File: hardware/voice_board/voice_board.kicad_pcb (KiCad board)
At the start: 2 copper layers, 131 parts, among them J1 Conn_02x06_Odd_Even, J10 Conn_01x02_Male, J2 Conn_02x02_Odd_Even, J3 Conn_02x02_Odd_Even, J4 Conn_01x02_Male, J5 Conn_02x03_Odd_Even, J6 Conn_02x02_Odd_Even, J7 Conn_02x02_Odd_Even, J8 Conn_02x02_Odd_Even, J9 Conn_02x02_Odd_Even, Q1 BC327, Q10 BC557, Q11 BC557, Q12 BC557, Q13 BC557, Q14 BC557, Q15 BC557, Q16 BC557, Q17 BC547, Q18 BC547, Q19 2N7000, Q2 BC557, Q20 2N7000, Q21 BC547, Q22 BC547, Q3 BC327, Q4 BC557, Q5 BC557, Q6 BC557, Q7 BC557, Q8 BC557, Q9 BC557, U1 TL074, U2 MCP4822, U3 LM324

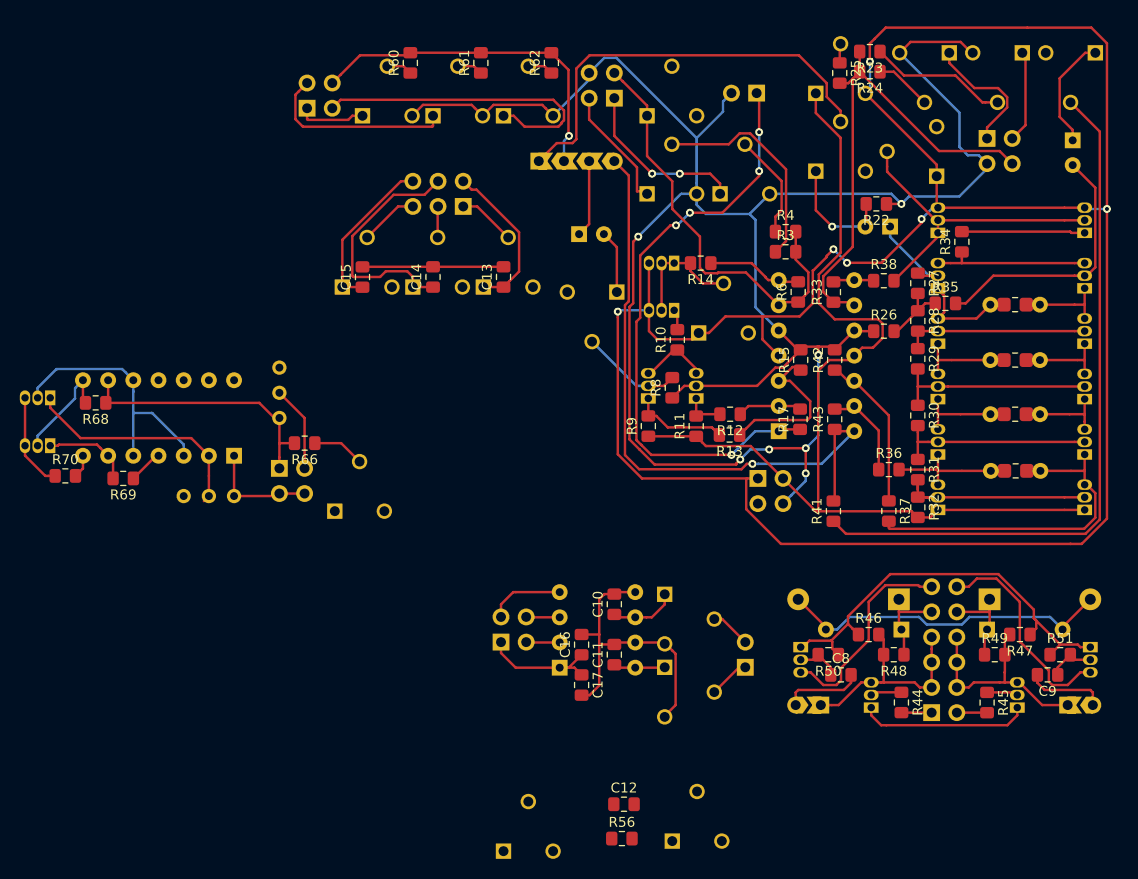
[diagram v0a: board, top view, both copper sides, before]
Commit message: silk screen final?
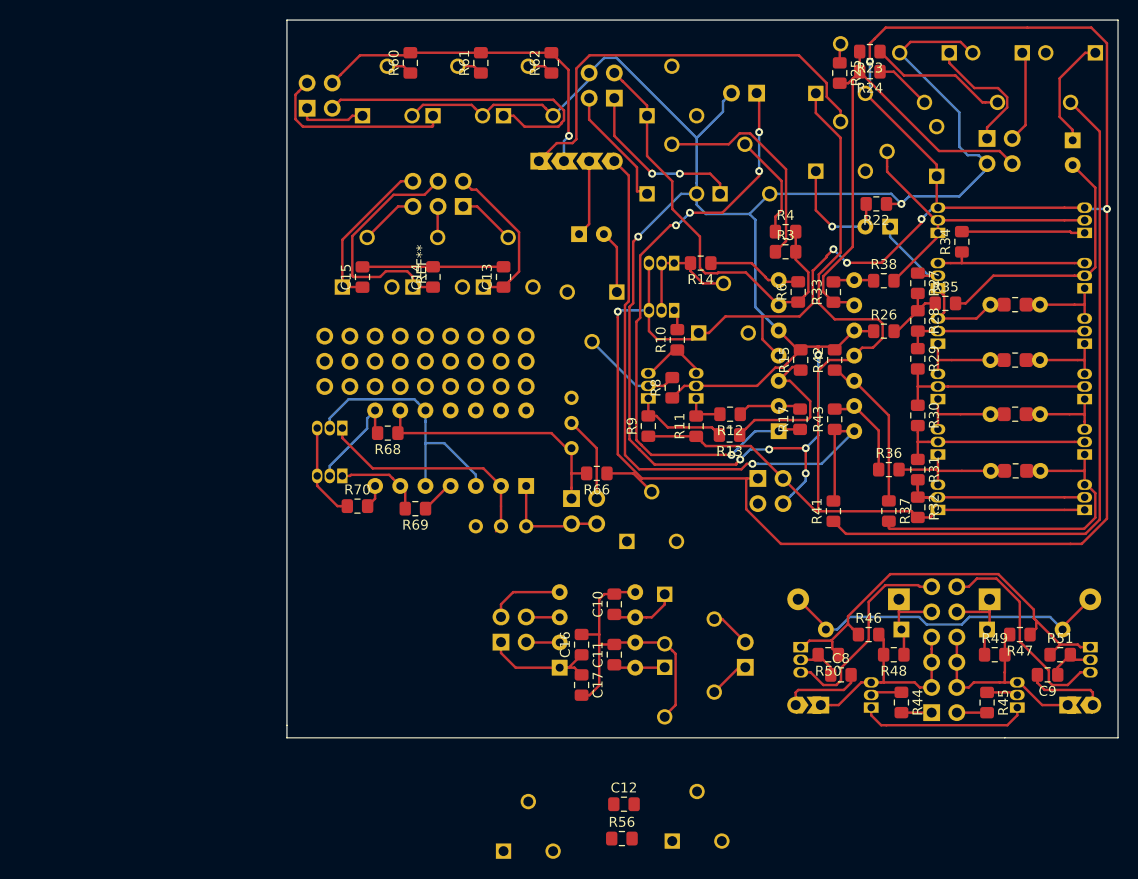
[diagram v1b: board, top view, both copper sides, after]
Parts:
- added G***: LOGO, windfisch:windfisch_smaller, B.Cu at (170.9, 95.2)
- added REF**: perfboard 3x9, footprints:perfboard 3x9, F.Cu at (176.4, 52.6)
- moved R68 29.6 mm to (173.5, 69.6)
- moved J7 29.6 mm to (192.0, 76.2)
- moved Q21 29.6 mm to (168.9, 73.9)
- moved Q22 29.6 mm to (168.9, 69.1)
- moved R66 29.6 mm to (194.6, 73.7)
- moved R67 29.6 mm to (192.0, 71.1)
- moved R69 29.6 mm to (176.3, 77.2)
- moved R70 29.6 mm to (170.4, 77.0)
- moved R71 29.6 mm to (187.5, 79.0)
- moved R72 29.6 mm to (197.6, 80.5)
- moved U3 29.6 mm to (187.5, 74.9)
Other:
- board outline added: 83.8 x 72.4 mm
- board text added: "(c) 2019 Florian Jung"
- board text added: "github.com/Windfisch/ analog-synth"
- board text added: "square_ctl"
- board text added: "voice board mk I"
- board text removed: "square_ctl buffer and sync"
